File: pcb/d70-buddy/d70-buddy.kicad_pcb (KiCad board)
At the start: 2 copper layers, 210 x 17.9 mm, 16 parts, among them J1 Conn_02x11_Top_Bottom, J2 Conn_02x04_Top_Bottom, SW1 SW_Push_LED_YELLOW, SW2 SW_Push_LED_GREEN, SW3 SW_Push_LED_BLUE, SW4 SW_Push_LED_WHITE, SW5 SW_Push_LED_RED, SW6 SW_Push_LED_WHITE, SW7 SW_Push_LED_GREEN

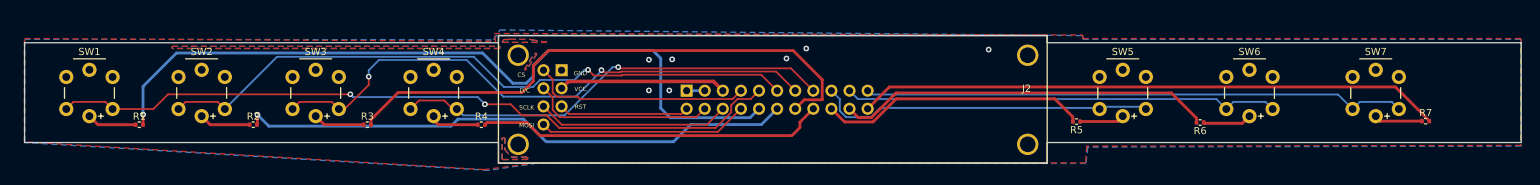
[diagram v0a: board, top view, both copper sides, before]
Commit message: Wip
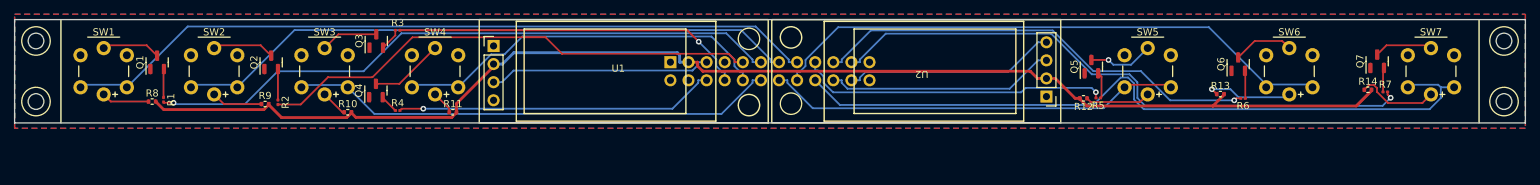
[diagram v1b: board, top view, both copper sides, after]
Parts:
- removed J2: Conn_02x04_Top_Bottom, lib:ELW2106AA
- added H1: MountingHole_2.2mm_M2, MountingHole:MountingHole_2.2mm_M2, F.Cu at (51.0, 102.8)
- added H2: MountingHole_2.2mm_M2, MountingHole:MountingHole_2.2mm_M2, F.Cu at (51.0, 111.2)
- added H3: MountingHole_2.2mm_M2, MountingHole:MountingHole_2.2mm_M2, F.Cu at (257.0, 102.8)
- added H4: MountingHole_2.2mm_M2, MountingHole:MountingHole_2.2mm_M2, F.Cu at (257.0, 111.2)
- added Q1: MBT2222A, Package_TO_SOT_SMD:SOT-23, F.Cu at (68.0, 105.8)
- added Q2: MBT2222A, Package_TO_SOT_SMD:SOT-23, F.Cu at (84.0, 105.8)
- added Q3: MBT2222A, Package_TO_SOT_SMD:SOT-23, F.Cu at (98.8, 102.8)
- added Q4: MBT2222A, Package_TO_SOT_SMD:SOT-23, F.Cu at (98.7, 109.7)
- added Q5: MBT2222A, Package_TO_SOT_SMD:SOT-23, F.Cu at (199.1, 106.3)
- added Q6: MBT2222A, Package_TO_SOT_SMD:SOT-23, F.Cu at (219.7, 106.0)
- added Q7: MBT2222A, Package_TO_SOT_SMD:SOT-23, F.Cu at (239.2, 105.6)
- added R10: 51, Resistor_SMD:R_0402_1005Metric, F.Cu at (94.8, 112.8)
- added R11: 51, Resistor_SMD:R_0402_1005Metric, F.Cu at (109.5, 112.8)
- added R12: 51, Resistor_SMD:R_0402_1005Metric, F.Cu at (198.0, 110.8)
- added R13: 51, Resistor_SMD:R_0402_1005Metric, F.Cu at (217.2, 110.2)
- added R14: 51, Resistor_SMD:R_0402_1005Metric, F.Cu at (237.9, 109.6)
- added R8: 51, Resistor_SMD:R_0402_1005Metric, F.Cu at (67.3, 111.2)
- added R9: 51, Resistor_SMD:R_0402_1005Metric, F.Cu at (83.2, 111.6)
- added U1: SSD1312_I2C_128x64, OLED SSD1312 KiCAD:OLED_SSD1312_I2C_0.96_No_Mounting_Holes, F.Cu at (133.4, 108.0)
- added U2: SSD1312_I2C_128x64, OLED SSD1312 KiCAD:OLED_SSD1312_I2C_0.96_No_Mounting_Holes, F.Cu at (174.6, 106.0)
- J1: value Conn_02x11_Top_Bottom -> Conn_02x12_Top_Bottom; footprint Connector_PinHeader_2.54mm:PinHeader_2x11_P2.54mm_Vertical -> Connector_PinHeader_2.54mm:PinHeader_2x12_P2.54mm_Vertical
- R1, R5: value 68 -> 25000; footprint Resistor_SMD:R_0402_1005Metric -> Resistor_SMD:R_0201_0603Metric
- R2, R3, R4, R6, R7: value 150 -> 25000; footprint Resistor_SMD:R_0402_1005Metric -> Resistor_SMD:R_0201_0603Metric
- SW2, SW7: value SW_Push_LED_GREEN -> SW_Push_LED_YELLOW
- SW3: value SW_Push_LED_BLUE -> SW_Push_LED_YELLOW
- SW4, SW6: value SW_Push_LED_WHITE -> SW_Push_LED_YELLOW
- SW5: value SW_Push_LED_RED -> SW_Push_LED_YELLOW
- moved R3 13.9 mm to (101.8, 101.2)
- moved R4 11.9 mm to (101.8, 112.5)
- moved SW7 11.0 mm to (246.8, 107.0)
- moved SW6 8.88 mm to (226.9, 107.0)
- moved R7 6.98 mm to (240.3, 109.9)
- moved R6 6.91 mm to (220.4, 110.8)
- moved SW5 6.80 mm to (207.0, 107.0)
- moved SW1 5.31 mm to (60.5, 107.0)
- moved SW2 5.06 mm to (76.0, 107.0)
- moved R1 4.88 mm to (68.9, 111.0), turned to -90 degrees
- moved R2 4.68 mm to (85.0, 111.3), turned to -90 degrees
- moved J1 4.60 mm to (140.0, 105.7)
- moved SW3 4.57 mm to (91.5, 107.0)
- moved R5 4.50 mm to (200.1, 110.8)
- moved SW4 3.54 mm to (107.0, 107.0)
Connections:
- J1 pad 10: /LED_1 -> /BTN_4
- J1 pad 11: /BTN_2 -> /LED_1
- J1 pad 12: /LED_2 -> /BTN_3
- J1 pad 13: /BTN_3 -> /BTN_2
- J1 pad 14: /LED_3 -> /BTN_5
- J1 pad 15: /BTN_4 -> /BTN_1
- J1 pad 16: /LED_4 -> /BTN_6
- J1 pad 17: /BTN_5 -> /LED_5
- J1 pad 18: /LED_5 -> /BTN_7
- J1 pad 19: /BTN_6 -> /LED_6
- J1 pad 2: /RST -> GND
- J1 pad 20: /LED_6 -> /SCL2
- J1 pad 21: /BTN_7 -> /LED_7
- J1 pad 22: /LED_7 -> /SDA2
- J1 pad 3: GND -> +3V3
- J1 pad 4: /D/C -> +5V
- J1 pad 5: VCC -> /SCL1
- J1 pad 6: /SCLK -> /LED_4
- J1 pad 7: /CS -> unconnected-(J1-Pad7)
- J1 pad 8: /MOSI -> /LED_3
- J1 pad 9: /BTN_1 -> /LED_2
- R1 pad 1: Net-(SW1-Pad4) -> Net-(Q1-Pad2)
- R2 pad 1: Net-(SW2-Pad4) -> Net-(R2-Pad1)
- R3 pad 1: Net-(SW3-Pad4) -> Net-(Q3-Pad2)
- R4 pad 1: Net-(SW4-Pad4) -> Net-(Q4-Pad2)
- R5 pad 1: Net-(SW5-Pad4) -> Net-(Q5-Pad2)
- R6 pad 1: Net-(SW6-Pad4) -> Net-(Q6-Pad2)
- R7 pad 1: Net-(SW7-Pad4) -> Net-(Q7-Pad2)
- SW1 pad 3: GND -> Net-(SW1-Pad3)
- SW2 pad 3: GND -> Net-(SW2-Pad3)
- SW2 pad 4: Net-(SW2-Pad4) -> Net-(R9-Pad1)
- SW3 pad 3: GND -> Net-(Q3-Pad3)
- SW3 pad 4: Net-(SW3-Pad4) -> Net-(R10-Pad1)
- SW4 pad 3: GND -> Net-(Q4-Pad3)
- SW4 pad 4: Net-(SW4-Pad4) -> Net-(R11-Pad1)
- SW5 pad 3: GND -> Net-(Q5-Pad3)
- SW5 pad 4: Net-(SW5-Pad4) -> Net-(R12-Pad1)
- SW6 pad 3: GND -> Net-(Q6-Pad3)
- SW6 pad 4: Net-(SW6-Pad4) -> Net-(R13-Pad1)
- SW7 pad 3: GND -> Net-(Q7-Pad3)
- SW7 pad 4: Net-(SW7-Pad4) -> Net-(R14-Pad1)
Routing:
- net +3V3: track 0.00 -> 184.9 mm
- net /SCL2: track 0.00 -> 32.3 mm
- net /SCL1: track 0.00 -> 31.3 mm
- net /CS: track 31.0 -> 0.00 mm
- net /SDA2: track 0.00 -> 29.8 mm
- net /MOSI: track 29.5 -> 0.00 mm
- net /LED_3: track 78.1 -> 49.7 mm, vias 0 -> 1
- net /SCLK: track 27.2 -> 0.00 mm
- net /BTN_7: track 76.4 -> 102.9 mm
- net /D/C: track 25.8 -> 0.00 mm
- net VCC: track 23.6 -> 0.00 mm
- net /BTN_6: track 61.3 -> 80.5 mm
- net /RST: track 18.3 -> 0.00 mm
- net /LED_1: track 106.8 -> 90.0 mm
- net Net-(R13-Pad1): track 0.00 -> 12.5 mm, vias 0 -> 1
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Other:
- board size 210 x 17.9 mm -> 212 x 14.5 mm
